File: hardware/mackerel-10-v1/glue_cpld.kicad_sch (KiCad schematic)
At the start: 18 parts, among them J1 Conn_02x05_Odd_Even, X1 50MHz, X2 50MHz

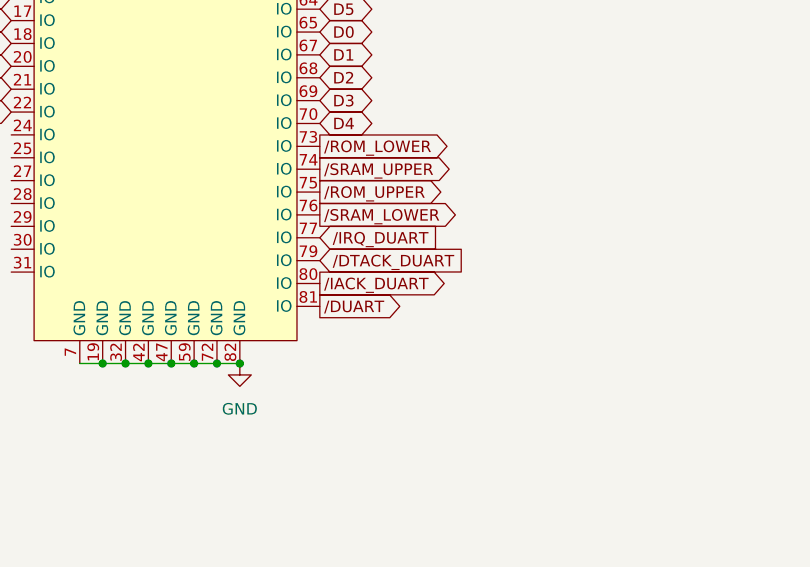
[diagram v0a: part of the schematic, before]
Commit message: Mostly routed except expansion
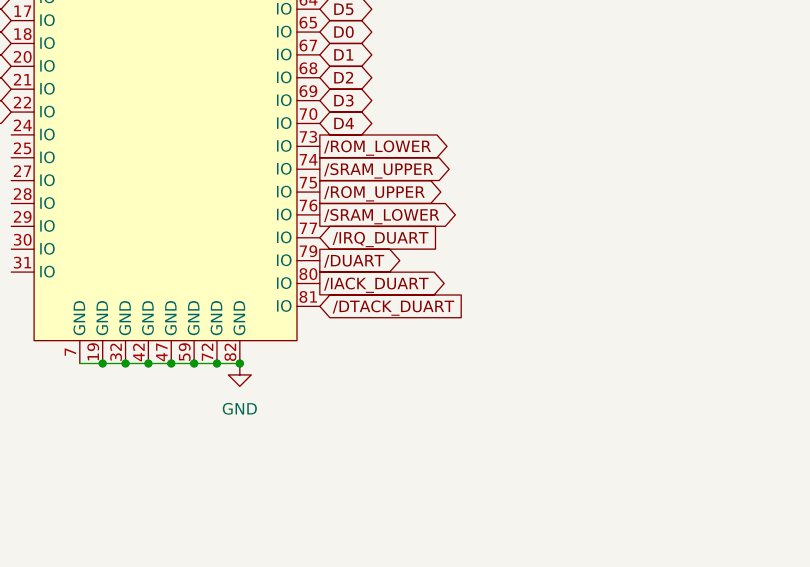
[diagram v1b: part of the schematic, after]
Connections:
- net /DTACK_DUART: now also U2.81 (IO); no longer U2.79 (IO)
- net /DUART: now also U2.79 (IO); no longer U2.81 (IO)
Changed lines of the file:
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@@
 	(global_label "{slash}DTACK_DUART"
 		(shape input)
-		(at 147.32 137.16 0)
-		(fields_autoplaced yes)
-		(effects
-			(font
-				(size 1.27 1.27)
-			)
-			(justify left)
-		)
-		(property "Intersheetrefs" "${INTERSHEET_REFS}"
-			(at 164.3962 137.16 0)
+		(at 147.32 142.24 0)
+		(fields_autoplaced yes)
+		(effects
+			(font
+				(size 1.27 1.27)
+			)
+			(justify left)
+		)
+		(property "Intersheetrefs" "${INTERSHEET_REFS}"
+			(at 164.3962 142.24 0)
 			(effects
 				(font
@@
 	(global_label "{slash}DUART"
 		(shape output)
-		(at 147.32 142.24 0)
-		(fields_autoplaced yes)
-		(effects
-			(font
-				(size 1.27 1.27)
-			)
-			(justify left)
-		)
-		(property "Intersheetrefs" "${INTERSHEET_REFS}"
-			(at 157.5624 142.24 0)
-			(effects
-				(font
+		(at 147.32 137.16 0)
+		(fields_autoplaced yes)
+		(effects
+			(font
+				(size 1.27 1.27)
+			)
+			(justify left)
+		)
+		(property "Intersheetrefs" "${INTERSHEET_REFS}"
+			(at 157.5624 137.16 0)
+			(effects
+				(font
